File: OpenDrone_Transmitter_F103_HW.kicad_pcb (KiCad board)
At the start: 2 copper layers, 57 x 32 mm, 78 parts, among them J1 Conn_01x03, J10 Conn_01x04, J11 Conn_01x03, J12 Conn_01x04, J13 Conn_01x02, J14 Conn_01x05, J15 Conn_01x02, J16 Conn_02x04_Odd_Even, J17 Conn_01x02, J18 Conn_01x02, J19 Conn_01x03, J2 Conn_01x05, J20 Conn_01x02, J21 Conn_01x02, J22 Conn_01x02, J3 Conn_01x03, J4 Conn_01x03, J5 Conn_01x03, J6 Conn_01x02, J7 Conn_01x02, J8 Conn_01x03, J9 Conn_01x03, SW1 RESET, U1 STM32F103C8Tx, U2 AMS1117-3.3, U3 TPS54331, Y2 Crystal_GND24

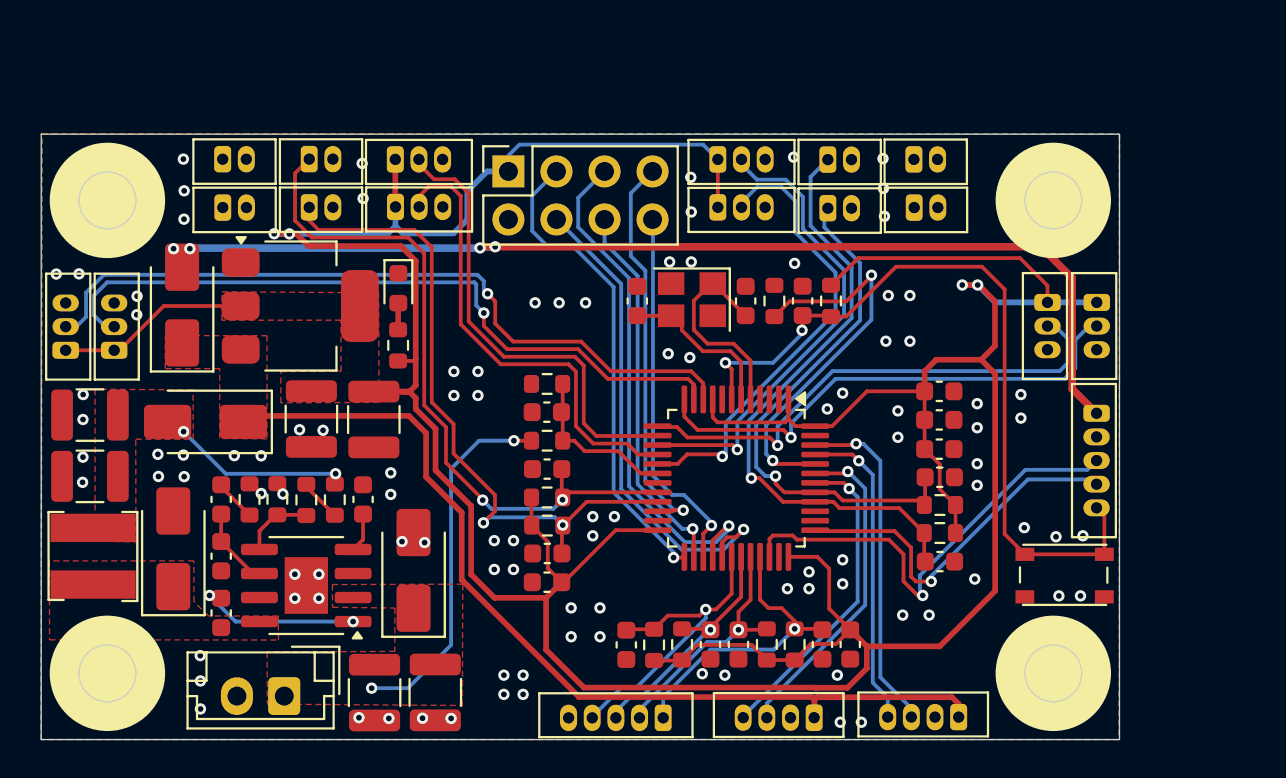
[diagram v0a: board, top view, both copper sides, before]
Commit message: update
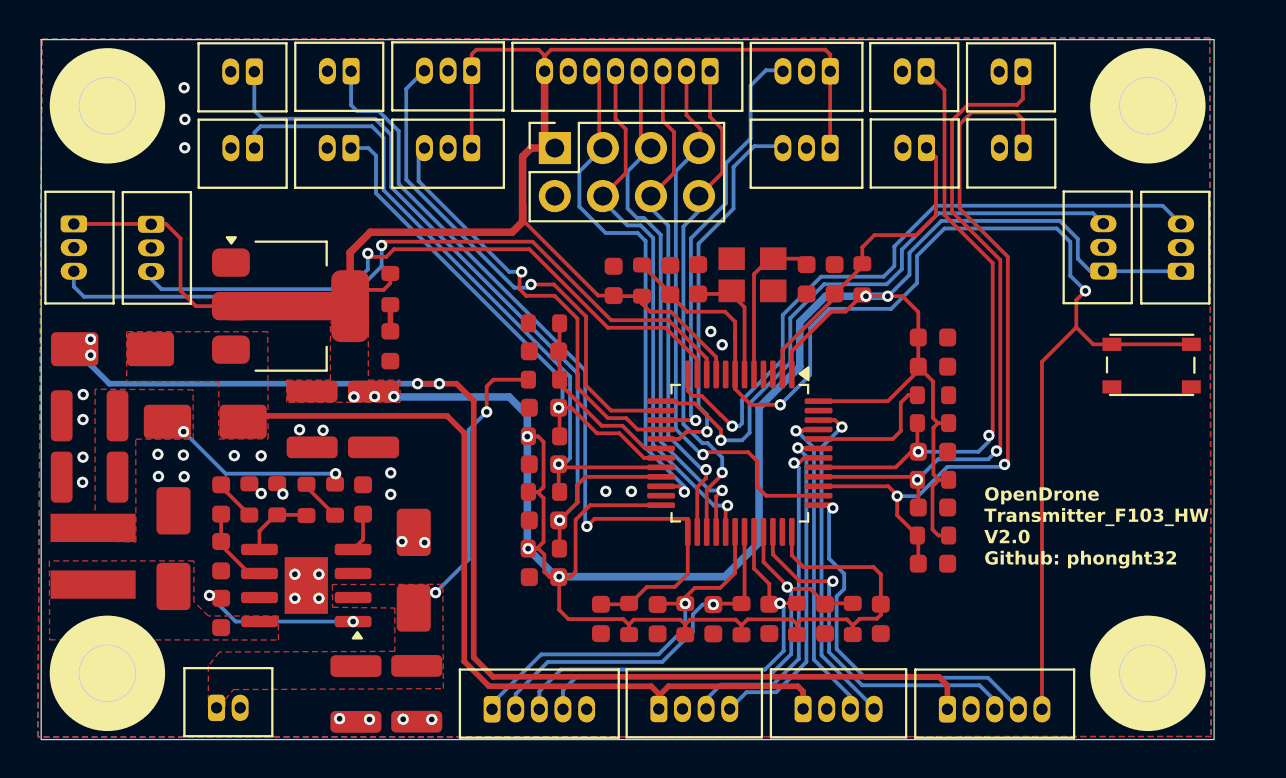
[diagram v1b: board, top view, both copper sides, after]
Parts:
- added C10: 100nF, KiCad-Lib:C_0603_1608Metric, F.Cu at (193.1, 102.7)
- added C21: 100nF, KiCad-Lib:C_0603_1608Metric, F.Cu at (210.6, 99.8)
- added C30: 100nF, KiCad-Lib:C_0603_1608Metric, F.Cu at (190.1, 91.5)
- added C31: 100nF, KiCad-Lib:C_0603_1608Metric, F.Cu at (205.4, 84.7)
- added J23: Conn_01x08, KiCad-Lib:Connector_ZH_1x08_P1.25mm_Vertical, F.Cu at (198.9, 73.7)
- added R18: 1k, KiCad-Lib:R_0603_1608Metric, F.Cu at (194.6, 102.7)
- added R19: 1k, KiCad-Lib:R_0603_1608Metric, F.Cu at (210.6, 98.3)
- added R20: 1k, KiCad-Lib:R_0603_1608Metric, F.Cu at (190.1, 93.1)
- added R21: 1k, KiCad-Lib:R_0603_1608Metric, F.Cu at (206.9, 84.7)
- C1, C2, C20, C4, C5, C9: footprint Capacitor_SMD:C_1210_3225Metric -> KiCad-Lib:C_1210_3225Metric
- C11, C12, C13, C14, C15, C16, C17, C18, C19, C22, C23, C24, C25, C26, C27, C28, C29, C3, C6, C7, C8: footprint Capacitor_SMD:C_0603_1608Metric -> KiCad-Lib:C_0603_1608Metric
- D1, D2, D3, D4: footprint Diode_SMD:D_SMA -> KiCad-Lib:D_SMA
- D5: footprint LED_SMD:LED_0603_1608Metric -> KiCad-Lib:LED_0603_1608Metric
- J1, J11, J19, J3, J4, J5, J8, J9: footprint Footprint:Connector_XH_1x03_P1.25mm_Vertical -> KiCad-Lib:Connector_ZH_1x03_P1.25mm_Vertical
- J10, J12: footprint Footprint:Connector_XH_1x04_P1.25mm_Vertical -> KiCad-Lib:Connector_ZH_1x04_P1.25mm_Vertical
- J13, J15, J17, J18, J20, J21, J22, J6: footprint Footprint:Connector_XH_1x02_P1.25mm_Vertical -> KiCad-Lib:Connector_ZH_1x02_P1.25mm_Vertical
- J14, J2: footprint Footprint:Connector_XH_1x05_P1.25mm_Vertical -> KiCad-Lib:Connector_ZH_1x05_P1.25mm_Vertical
- J7: footprint Connector_JST:JST_EH_B2B-EH-A_1x02_P2.50mm_Vertical -> KiCad-Lib:Connector_ZH_1x02_P1.25mm_Vertical
- L1: footprint Footprint:Inductor_SMD_4D28 -> KiCad-Lib:Inductor_SMD_4D28
- R1, R10, R11, R12, R13, R14, R15, R16, R17, R2, R3, R4, R5, R6, R7, R8, R9: footprint Resistor_SMD:R_0603_1608Metric -> KiCad-Lib:R_0603_1608Metric
- SW1: footprint Footprint:Button_SMD_4.2x3.3x2.5mm -> KiCad-Lib:Button_SMD_4.2x3.3x2.5mm
- U3: footprint Package_SO:SOIC-8-1EP_3.9x4.9mm_P1.27mm_EP2.29x3mm -> KiCad-Lib:SOIC-8-1EP_3.9x4.9mm_P1.27mm_EP2.29x3mm
- U4: footprint Footprint:Board -> Proj-Lib:Board
- Y2: footprint Crystal:Crystal_SMD_3225-4Pin_3.2x2.5mm -> KiCad-Lib:Crystal_SMD_3225-4Pin_3.2x2.5mm
- moved C3 18.2 mm to (193.8, 84.8), turned to 90 degrees
- moved J2 17.5 mm to (211.4, 107.5), turned to 0 degrees
- moved SW1 12.0 mm to (222.2, 89.3)
- moved J15 11.3 mm to (215.4, 73.8), turned to 180 degrees
- moved R3 10.0 mm to (195.3, 84.8), turned to 90 degrees
- moved R4 9.75 mm to (210.6, 90.9), turned to 180 degrees
- moved J14 9.06 mm to (187.3, 107.5), turned to 0 degrees
- moved J18 8.90 mm to (210.3, 73.7), turned to 180 degrees
- moved J10 8.24 mm to (203.8, 107.5), turned to 0 degrees
- moved J6 8.23 mm to (179.9, 73.7), turned to 180 degrees
- moved J12 8.22 mm to (196.2, 107.5), turned to 0 degrees
- moved J17 7.74 mm to (174.8, 73.8), turned to 180 degrees
- moved J1 7.55 mm to (205.2, 73.7), turned to 180 degrees
- moved J20 7.47 mm to (179.9, 77.8), turned to 180 degrees
- moved C6 7.08 mm to (196.8, 84.8)
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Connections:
- net SWITCH1 renamed PB2
- net SWITCH2 renamed PB4
- net SWITCH3 renamed PB10
- net SWITCH4 renamed PB5
- J1 pad 2: VOLUME_2 -> GND
- J1 pad 3: GND -> VOLUME_2
- J10 pad 3: I2C1_SDA -> I2C1_SCL
- J10 pad 4: I2C1_SCL -> I2C1_SDA
- J11 pad 2: VOLUME_4 -> GND
- J11 pad 3: GND -> VOLUME_4
- J12 pad 3: UART1_RX -> UART1_TX
- J12 pad 4: UART1_TX -> UART1_RX
- J14 pad 1: BUTTON4 -> BUTTON1
- J14 pad 2: BUTTON3 -> BUTTON2
- J14 pad 3: BUTTON2 -> BUTTON3
- J14 pad 4: BUTTON1 -> BUTTON4
- J19 pad 2: RIGHT_JOYSTICK_IN1 -> GND
- J19 pad 3: GND -> RIGHT_JOYSTICK_IN1
- J20 pad 1: unconnected-(J20-Pin_1-Pad1) -> PB1
- J20 pad 2: unconnected-(J20-Pin_2-Pad2) -> GND
- J21 pad 1: unconnected-(J21-Pin_1-Pad1) -> PB3
- J21 pad 2: unconnected-(J21-Pin_2-Pad2) -> GND
- J22 pad 1: unconnected-(J22-Pin_1-Pad1) -> PC13
- J22 pad 2: unconnected-(J22-Pin_2-Pad2) -> GND
- J3 pad 2: LEFT_JOYSTICK_IN1 -> GND
- J3 pad 3: GND -> LEFT_JOYSTICK_IN1
- J4 pad 2: LEFT_JOYSTICK_IN2 -> GND
- J4 pad 3: GND -> LEFT_JOYSTICK_IN2
- J5 pad 2: RIGHT_JOYSTICK_IN2 -> GND
- J5 pad 3: GND -> RIGHT_JOYSTICK_IN2
- J6 pad 1: unconnected-(J6-Pin_1-Pad1) -> PB12
- J6 pad 2: unconnected-(J6-Pin_2-Pad2) -> GND
- J8 pad 2: VOLUME_1 -> GND
- J8 pad 3: GND -> VOLUME_1
- J9 pad 2: VOLUME_3 -> GND
- J9 pad 3: GND -> VOLUME_3
- U1 pad 19: unconnected-(U1-PB1-Pad19) -> PB1
- U1 pad 2: unconnected-(U1-PC13-Pad2) -> PC13
- U1 pad 22: NRF24_IRQ -> NRF24_CS
- U1 pad 25: NRF24_CS -> PB12
- U1 pad 38: unconnected-(U1-PA15-Pad38) -> NRF24_IRQ
- U1 pad 39: unconnected-(U1-PB3-Pad39) -> PB3
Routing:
- net PB12: track 0.00 -> 43.6 mm, vias 0 -> 1
- net PB3: track 0.00 -> 39.2 mm, vias 0 -> 2
- net +3V3: track 205.0 -> 240.6 mm, vias 4 -> 8
- net PB1: track 0.00 -> 27.0 mm, vias 0 -> 1
- net STM32_RESET: track 41.7 -> 66.9 mm
- net PC13: track 0.00 -> 16.7 mm
- net Net-(U1-BOOT0): track 20.6 -> 7.06 mm, vias 2 -> 0
- net BUTTON3: track 13.3 -> 23.0 mm
- net BUTTON4: track 16.1 -> 25.1 mm
- net RIGHT_JOYSTICK_IN1: track 26.9 -> 35.6 mm
- net NRF24_IRQ: track 21.2 -> 29.7 mm
- net PB10: track 35.5 -> 43.1 mm, vias 2 -> 1
- net 5V_DEBUGGER: track 56.7 -> 64.1 mm
- net NRF24_MISO: track 19.7 -> 26.8 mm
- net NRF24_CLK: track 20.1 -> 26.6 mm
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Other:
- board size 57 x 32 mm -> 62 x 37 mm
- board text added: "+"
- board text added: "-"
- board text added: "A0"
- board text added: "A1"
- board text added: "A3"
- board text added: "A4"
- board text added: "A5"
- board text added: "A6"
- board text added: "A7"
- board text added: "B1"
- board text added: "B10"
- board text added: "B12"
- board text added: "B2"
- board text added: "B3"
- board text added: "B4"
- board text added: "B5"
- board text added: "C13"
- board text added: "G"
- board text added: "MI"
- board text added: "MO"
- board text added: "OpenDrone Transmitter_F103_HW V2.0 Github: phonght32"
- board text added: "R1"
- board text added: "T1"
- board text removed: "LIN1"
- board text removed: "LIN2"
- board text removed: "OpenDrone Transmitter_F103_HW V1.0 Github: phonght32"
- board text removed: "RIN1"
- board text removed: "RIN2"
- board text removed: "RX1"
- board text removed: "SW1"
- board text removed: "SW2"
- board text removed: "SW3"
- board text removed: "SW4"
- board text removed: "TX1"
- board text removed: "VBAT"
- board text removed: "VOL1"
- board text removed: "VOL2"
- board text removed: "VOL3"
- board text removed: "VOL4"
